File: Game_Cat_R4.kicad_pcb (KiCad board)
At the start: 2 copper layers, 160 x 60 mm, 195 parts, among them J1 USB_C, J2 CAN, J3 Joystick, J5 CORTEX-SWD, J6 UART, J7 PWM, J8 DM3AT-SF-PEJM5, Q1 2N2907, Q10 2N7002, Q2 2N2907, Q3 2N7002, Q4 FDN340P, Q5 NTR1P02LT1, Q6 BS138, Q7 BS138, Q8 BS138, Q9 BS138, SW1 A, SW2 B, SW3 X, SW4 Y, SW5 L, SW6 R, SW7 Reset, SW8 SW_SPDT, U1 ATSAMD21G18A, U10 LM61, U11 MCP73831, U12 TPS54231, U13 TCAN337GDR, U2 TPD2E2U06, U3 MCP2518FD, U5 24LC512, U6 23KXX, U7 74HC4051, U8 MMA8452Q, U9 SST26VF032B, Y1 20Mhz, Y2 Crystal_GND3

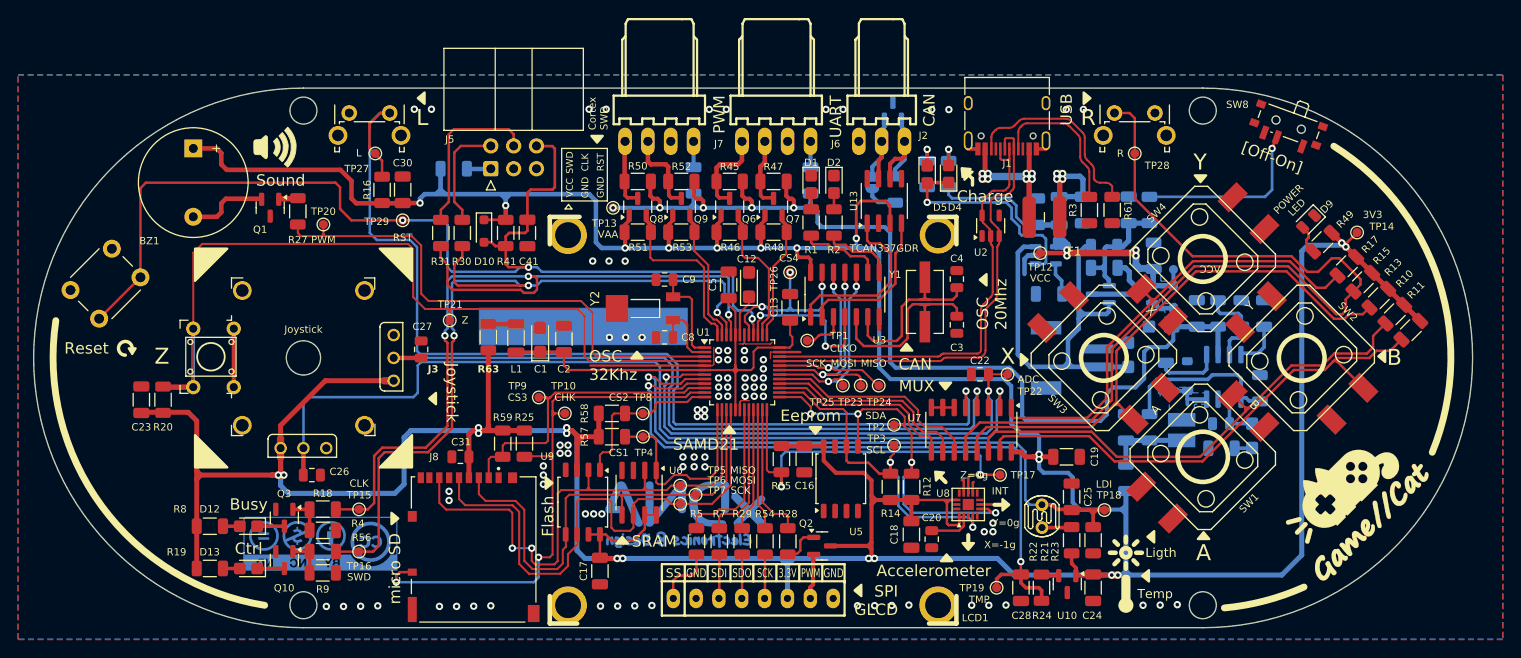
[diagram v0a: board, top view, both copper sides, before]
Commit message: 03/12/26/Update BOM & Models VRML
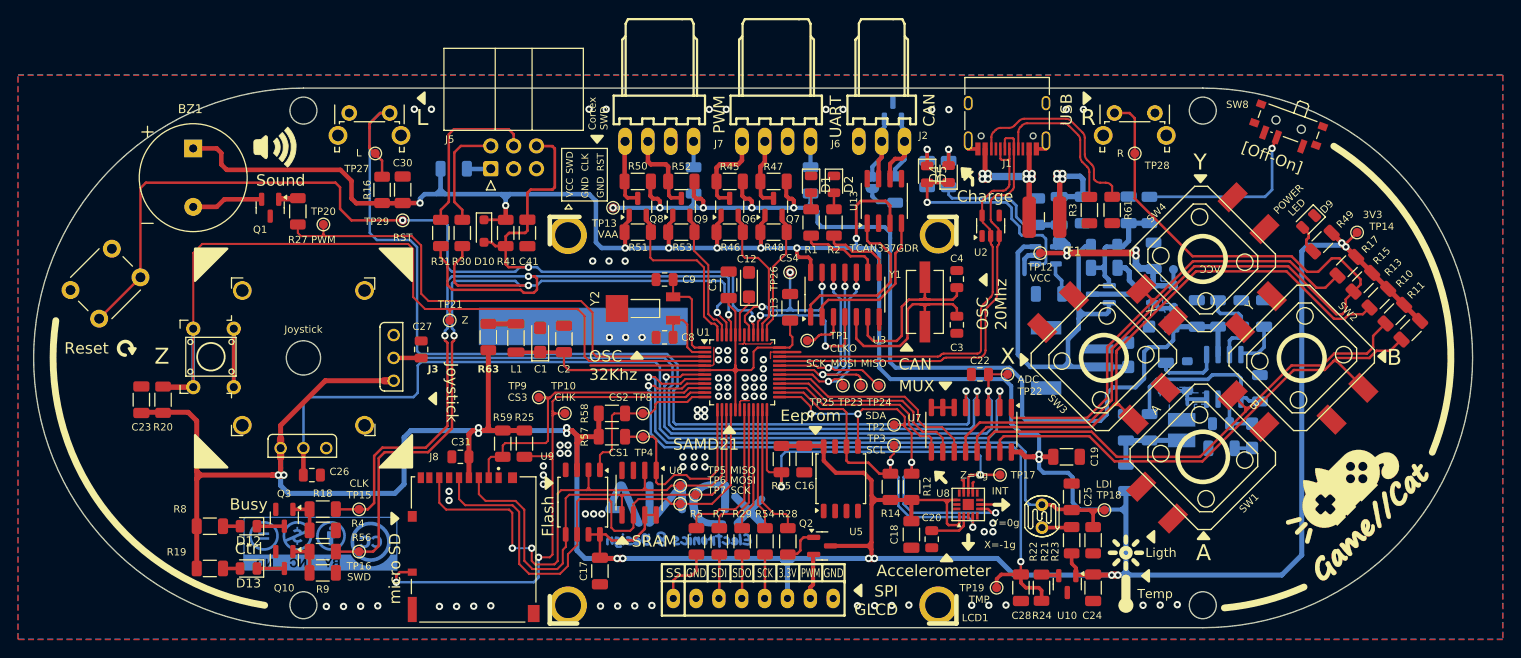
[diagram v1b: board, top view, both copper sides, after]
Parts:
- BZ1: footprint Buzzer_Beeper:Buzzer_12x9.5RM7.6 -> x_Buzzer:AT_1224_TWT_5V_2_R
- C1: value 10uF -> 4.7uF
- D1, D12, D13, D2, D4, D5: footprint LED_SMD:LED_0805_2012Metric_Castellated -> LED_SMD:LED_0805_2012Metric
- F1: value 500mA -> 2016L100PR
- L1: value BLM18PG471 -> FB321611T
- Q1, Q2: value 2N2907 -> MMBT2907A
- Q6, Q7, Q8, Q9: value BS138 -> BSS138
- U10: value LM61 -> TC1046
- U3: value MCP2518FD -> MCP2518FDT
- U5: value 24LC512 -> 24CSM01
- U6: value 23KXX -> 23K256
- U9: value SST26VF032B -> AT25DF641A
- Y1: value 20Mhz -> 4Mhz
- moved BZ1 3.25 mm to (67.7, 80.0), turned to 0 degrees
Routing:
- net Net-(BZ1-+): track 9.03 -> 7.96 mm
